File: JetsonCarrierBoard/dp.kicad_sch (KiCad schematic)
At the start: 0 parts

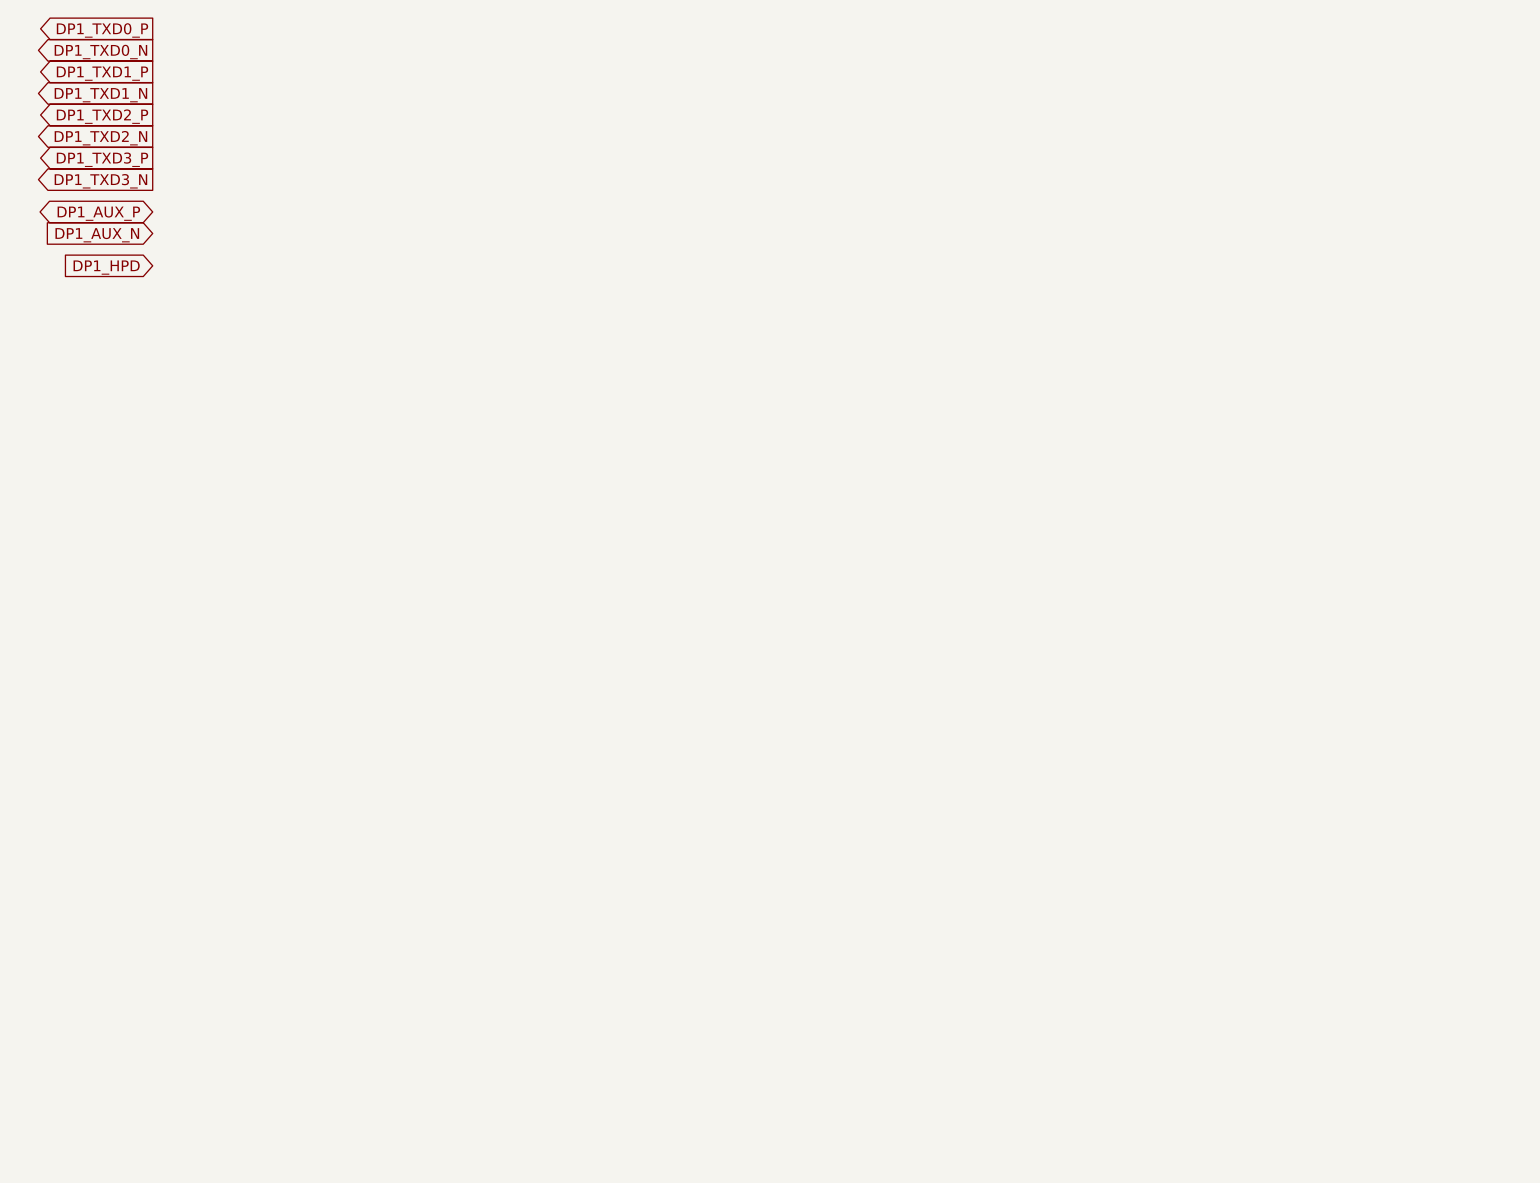
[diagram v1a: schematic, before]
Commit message: Small changes
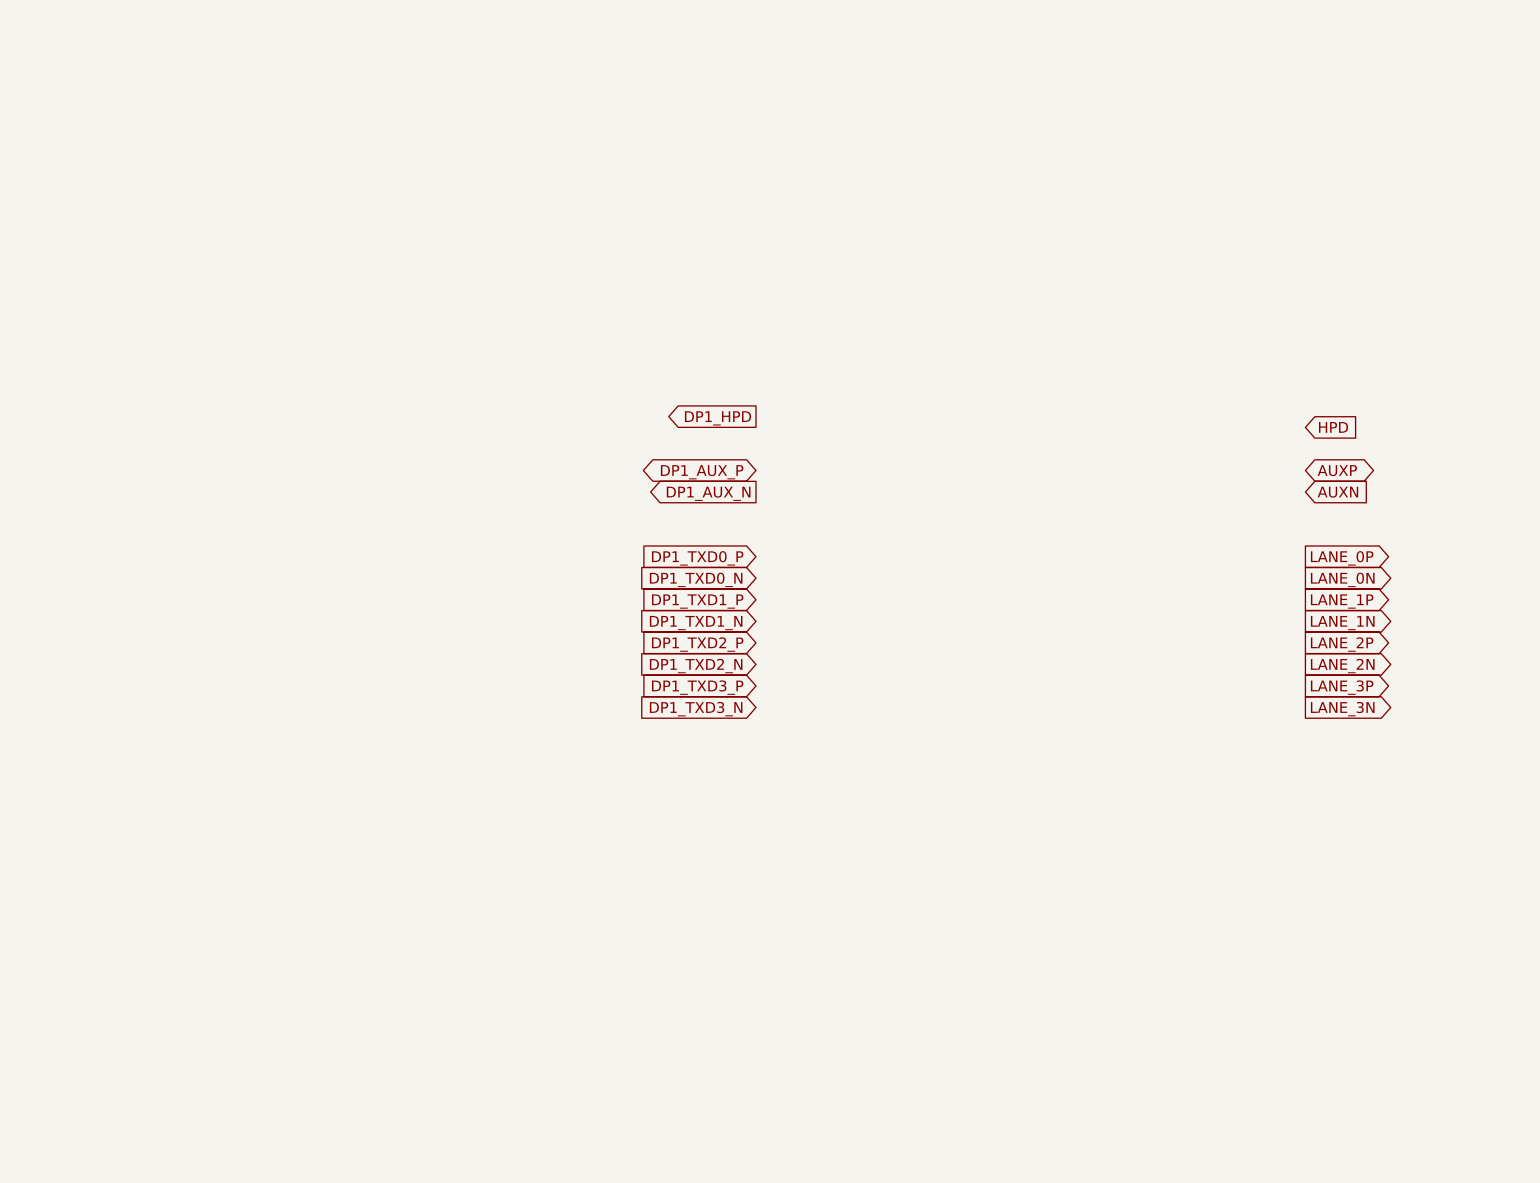
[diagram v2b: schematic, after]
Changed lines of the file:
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@@
 (kicad_sch (version 20211123) (generator eeschema)
   (paper "A4")
-  (global_label "DP1_AUX_P" (shape bidirectional) (at 35.56 43.18 180) (fields_autoplaced)
+  (global_label "LANE_2P" (shape output) (at 171.45 93.98 0) (fields_autoplaced)
+    (effects (font (size 1.27 1.27)) (justify left))
+    (property "Intersheet References" "${INTERSHEET_REFS}" (id 0) (at 181.9064 93.9006 0)
+      (effects (font (size 1.27 1.27)) (justify left) hide)
+    )
+  )
+  (global_label "DP1_AUX_P" (shape bidirectional) (at 106.68 73.66 180) (fields_autoplaced)
     (effects (font (size 1.27 1.27)) (justify right))
-    (property "Intersheet References" "${INTERSHEET_REFS}" (id 0) (at 22.5636 43.1006 0)
+    (property "Intersheet References" "${INTERSHEET_REFS}" (id 0) (at 93.6836 73.5806 0)
       (effects (font (size 1.27 1.27)) (justify right) hide)
     )
   )
-  (global_label "DP1_TXD3_P" (shape output) (at 35.56 36.83 180) (fields_autoplaced)
+  (global_label "DP1_TXD3_P" (shape input) (at 106.68 99.06 180) (fields_autoplaced)
     (effects (font (size 1.27 1.27)) (justify right))
-    (property "Intersheet References" "${INTERSHEET_REFS}" (id 0) (at 21.5355 36.7506 0)
+    (property "Intersheet References" "${INTERSHEET_REFS}" (id 0) (at 92.6555 98.9806 0)
       (effects (font (size 1.27 1.27)) (justify right) hide)
     )
   )
-  (global_label "DP1_TXD2_N" (shape output) (at 35.56 34.29 180) (fields_autoplaced)
+  (global_label "DP1_TXD2_N" (shape input) (at 106.68 96.52 180) (fields_autoplaced)
     (effects (font (size 1.27 1.27)) (justify right))
-    (property "Intersheet References" "${INTERSHEET_REFS}" (id 0) (at 21.475 34.2106 0)
+    (property "Intersheet References" "${INTERSHEET_REFS}" (id 0) (at 92.595 96.4406 0)
       (effects (font (size 1.27 1.27)) (justify right) hide)
     )
   )
-  (global_label "DP1_TXD2_P" (shape output) (at 35.56 31.75 180) (fields_autoplaced)
+  (global_label "DP1_TXD2_P" (shape input) (at 106.68 93.98 180) (fields_autoplaced)
     (effects (font (size 1.27 1.27)) (justify right))
-    (property "Intersheet References" "${INTERSHEET_REFS}" (id 0) (at 21.5355 31.6706 0)
+    (property "Intersheet References" "${INTERSHEET_REFS}" (id 0) (at 92.6555 93.9006 0)
       (effects (font (size 1.27 1.27)) (justify right) hide)
     )
   )
-  (global_label "DP1_AUX_N" (shape input) (at 35.56 45.72 180) (fields_autoplaced)
+  (global_label "LANE_1N" (shape output) (at 171.45 91.44 0) (fields_autoplaced)
+    (effects (font (size 1.27 1.27)) (justify left))
+    (property "Intersheet References" "${INTERSHEET_REFS}" (id 0) (at 181.9669 91.3606 0)
+      (effects (font (size 1.27 1.27)) (justify left) hide)
+    )
+  )
+  (global_label "DP1_AUX_N" (shape output) (at 106.68 76.2 180) (fields_autoplaced)
     (effects (font (size 1.27 1.27)) (justify right))
-    (property "Intersheet References" "${INTERSHEET_REFS}" (id 0) (at 22.5031 45.6406 0)
+    (property "Intersheet References" "${INTERSHEET_REFS}" (id 0) (at 93.6231 76.1206 0)
       (effects (font (size 1.27 1.27)) (justify right) hide)
     )
   )
-  (global_label "DP1_TXD3_N" (shape output) (at 35.56 39.37 180) (fields_autoplaced)
+  (global_label "DP1_TXD3_N" (shape input) (at 106.68 101.6 180) (fields_autoplaced)
     (effects (font (size 1.27 1.27)) (justify right))
-    (property "Intersheet References" "${INTERSHEET_REFS}" (id 0) (at 21.475 39.2906 0)
+    (property "Intersheet References" "${INTERSHEET_REFS}" (id 0) (at 92.595 101.5206 0)
       (effects (font (size 1.27 1.27)) (justify right) hide)
     )
   )
-  (global_label "DP1_TXD1_N" (shape output) (at 35.56 29.21 180) (fields_autoplaced)
+  (global_label "DP1_TXD1_N" (shape input) (at 106.68 91.44 180) (fields_autoplaced)
     (effects (font (size 1.27 1.27)) (justify right))
-    (property "Intersheet References" "${INTERSHEET_REFS}" (id 0) (at 21.475 29.1306 0)
+    (property "Intersheet References" "${INTERSHEET_REFS}" (id 0) (at 92.595 91.3606 0)
       (effects (font (size 1.27 1.27)) (justify right) hide)
     )
   )
-  (global_label "DP1_TXD1_P" (shape output) (at 35.56 26.67 180) (fields_autoplaced)
+  (global_label "AUXP" (shape bidirectional) (at 171.45 73.66 0) (fields_autoplaced)
+    (effects (font (size 1.27 1.27)) (justify left))
+    (property "Intersheet References" "${INTERSHEET_REFS}" (id 0) (at 178.7617 73.7394 0)
+      (effects (font (size 1.27 1.27)) (justify left) hide)
+    )
+  )
+  (global_label "DP1_TXD1_P" (shape input) (at 106.68 88.9 180) (fields_autoplaced)
     (effects (font (size 1.27 1.27)) (justify right))
-    (property "Intersheet References" "${INTERSHEET_REFS}" (id 0) (at 21.5355 26.5906 0)
+    (property "Intersheet References" "${INTERSHEET_REFS}" (id 0) (at 92.6555 88.8206 0)
       (effects (font (size 1.27 1.27)) (justify right) hide)
     )
   )
-  (global_label "DP1_HPD" (shape input) (at 35.56 49.53 180) (fields_autoplaced)
+  (global_label "LANE_1P" (shape output) (at 171.45 88.9 0) (fields_autoplaced)
+    (effects (font (size 1.27 1.27)) (justify left))
+    (property "Intersheet References" "${INTERSHEET_REFS}" (id 0) (at 181.9064 88.8206 0)
+      (effects (font (size 1.27 1.27)) (justify left) hide)
+    )
+  )
+  (global_label "LANE_3P" (shape output) (at 171.45 99.06 0) (fields_autoplaced)
+    (effects (font (size 1.27 1.27)) (justify left))
+    (property "Intersheet References" "${INTERSHEET_REFS}" (id 0) (at 181.9064 98.9806 0)
+      (effects (font (size 1.27 1.27)) (justify left) hide)
+    )
+  )
+  (global_label "AUXN" (shape input) (at 171.45 76.2 0) (fields_autoplaced)
+    (effects (font (size 1.27 1.27)) (justify left))
+    (property "Intersheet References" "${INTERSHEET_REFS}" (id 0) (at 178.8221 76.1206 0)
+      (effects (font (size 1.27 1.27)) (justify left) hide)
+    )
+  )
+  (global_label "HPD" (shape input) (at 171.45 68.58 0) (fields_autoplaced)
+    (effects (font (size 1.27 1.27)) (justify left))
+    (property "Intersheet References" "${INTERSHEET_REFS}" (id 0) (at 177.7336 68.5006 0)
+      (effects (font (size 1.27 1.27)) (justify left) hide)
+    )
+  )
+  (global_label "DP1_HPD" (shape output) (at 106.68 67.31 180) (fields_autoplaced)
     (effects (font (size 1.27 1.27)) (justify right))
-    (property "Intersheet References" "${INTERSHEET_REFS}" (id 0) (at 24.5593 49.4506 0)
+    (property "Intersheet References" "${INTERSHEET_REFS}" (id 0) (at 95.6793 67.2306 0)
       (effects (font (size 1.27 1.27)) (justify right) hide)
     )
   )
-  (global_label "DP1_TXD0_N" (shape output) (at 35.56 24.13 180) (fields_autoplaced)
+  (global_label "DP1_TXD0_N" (shape input) (at 106.68 86.36 180) (fields_autoplaced)
     (effects (font (size 1.27 1.27)) (justify right))
-    (property "Intersheet References" "${INTERSHEET_REFS}" (id 0) (at 21.475 24.0506 0)
+    (property "Intersheet References" "${INTERSHEET_REFS}" (id 0) (at 92.595 86.2806 0)
       (effects (font (size 1.27 1.27)) (justify right) hide)
     )
   )
-  (global_label "DP1_TXD0_P" (shape output) (at 35.56 21.59 180) (fields_autoplaced)
+  (global_label "LANE_3N" (shape output) (at 171.45 101.6 0) (fields_autoplaced)
+    (effects (font (size 1.27 1.27)) (justify left))
+    (property "Intersheet References" "${INTERSHEET_REFS}" (id 0) (at 181.9669 101.5206 0)
+      (effects (font (size 1.27 1.27)) (justify left) hide)
+    )
+  )
+  (global_label "DP1_TXD0_P" (shape input) (at 106.68 83.82 180) (fields_autoplaced)
     (effects (font (size 1.27 1.27)) (justify right))
-    (property "Intersheet References" "${INTERSHEET_REFS}" (id 0) (at 21.5355 21.5106 0)
+    (property "Intersheet References" "${INTERSHEET_REFS}" (id 0) (at 92.6555 83.7406 0)
       (effects (font (size 1.27 1.27)) (justify right) hide)
     )
   )
+  (global_label "LANE_2N" (shape output) (at 171.45 96.52 0) (fields_autoplaced)
+    (effects (font (size 1.27 1.27)) (justify left))
+    (property "Intersheet References" "${INTERSHEET_REFS}" (id 0) (at 181.9669 96.4406 0)
+      (effects (font (size 1.27 1.27)) (justify left) hide)
+    )
+  )
+  (global_label "LANE_0P" (shape output) (at 171.45 83.82 0) (fields_autoplaced)
+    (effects (font (size 1.27 1.27)) (justify left))
+    (property "Intersheet References" "${INTERSHEET_REFS}" (id 0) (at 181.9064 83.7406 0)
+      (effects (font (size 1.27 1.27)) (justify left) hide)
+    )
+  )
+  (global_label "LANE_0N" (shape output) (at 171.45 86.36 0) (fields_autoplaced)
+    (effects (font (size 1.27 1.27)) (justify left))
+    (property "Intersheet References" "${INTERSHEET_REFS}" (id 0) (at 181.9669 86.2806 0)
+      (effects (font (size 1.27 1.27)) (justify left) hide)
+    )
+  )

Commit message: Finished Basic DP wiring
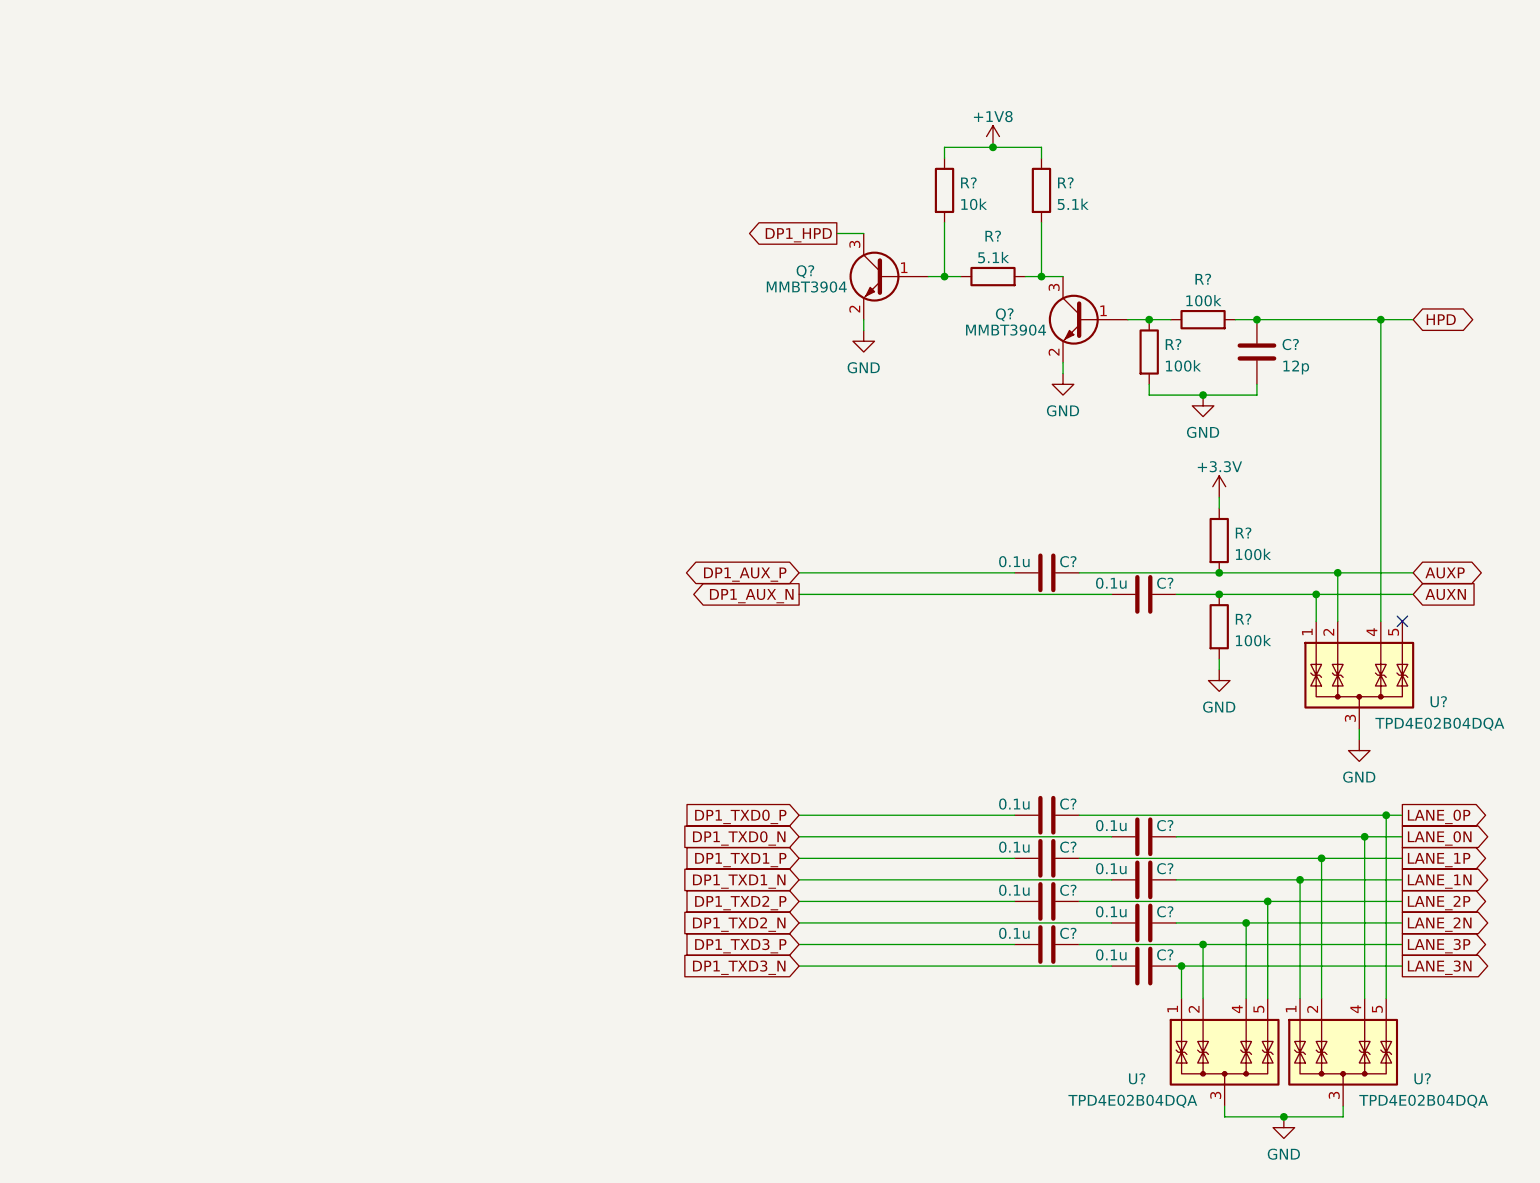
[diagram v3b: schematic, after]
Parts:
- added C?: 12p, symbol Device:C
- added C? (x10): 0.1u, symbol Device:C
- added Q? (x2): MMBT3904, Package_TO_SOT_SMD:SOT-23, symbol Transistor_BJT:MMBT3904
- added R? (x2): 5.1k, symbol Device:R
- added R? (x4): 100k, symbol Device:R
- added R?: 10k, symbol Device:R
- added U? (x3): TPD4E02B04DQA, Package_SON:USON-10_2.5x1.0mm_P0.5mm, symbol Power_Protection:TPD4E02B04DQA
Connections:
- net AUXN: now also C?.2, R?.1, U?.1 (IO1)
- net AUXP: now also C?.2, R?.2, U?.2 (IO2)
- net DP1_AUX_N: now also C?.1
- net DP1_AUX_P: now also C?.1
- net DP1_HPD: now also Q?.3 (C)
- net DP1_TXD0_N: now also C?.1
- net DP1_TXD0_P: now also C?.1
- net DP1_TXD1_N: now also C?.1
- net DP1_TXD1_P: now also C?.1
- net DP1_TXD2_N: now also C?.1
- net DP1_TXD2_P: now also C?.1
- net DP1_TXD3_N: now also C?.1
- net DP1_TXD3_P: now also C?.1
- net HPD: now also C?.1, R?.2, U?.4 (IO3)
- net LANE_0N: now also C?.2, U?.4 (IO3)
- net LANE_0P: now also C?.2, U?.5 (IO4)
- net LANE_1N: now also C?.2, U?.1 (IO1)
- net LANE_1P: now also C?.2, U?.2 (IO2)
- net LANE_2N: now also C?.2, U?.4 (IO3)
- net LANE_2P: now also C?.2, U?.5 (IO4)
- net LANE_3N: now also C?.2, U?.1 (IO1)
- net LANE_3P: now also C?.2, U?.2 (IO2)
- new net: Q?.3 (C), R?.2, R?.2
- new net: Q?.1 (B), R?.1, R?.2
- new net: Q?.1 (B), R?.1, R?.1
- new net +1V8: R?.1, R?.1
- new net +3V3: R?.1
- new net GND: C?.2, Q?.2 (E), Q?.2 (E), R?.2, R?.2, U?.3 (G), U?.3 (G), U?.3 (G), U?.8 (G), U?.8 (G), U?.8 (G)
- no-connect marks 0 -> 1
